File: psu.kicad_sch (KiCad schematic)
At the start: 70 parts, among them J3 Screw_Terminal_01x03, J4 Screw_Terminal_01x02, U14 ADP7182AUJZ, U15 AZ1117-ADJ, U16 AZ1117-ADJ, U19 ADP7182AUJZ, U2 AZ1117-ADJ

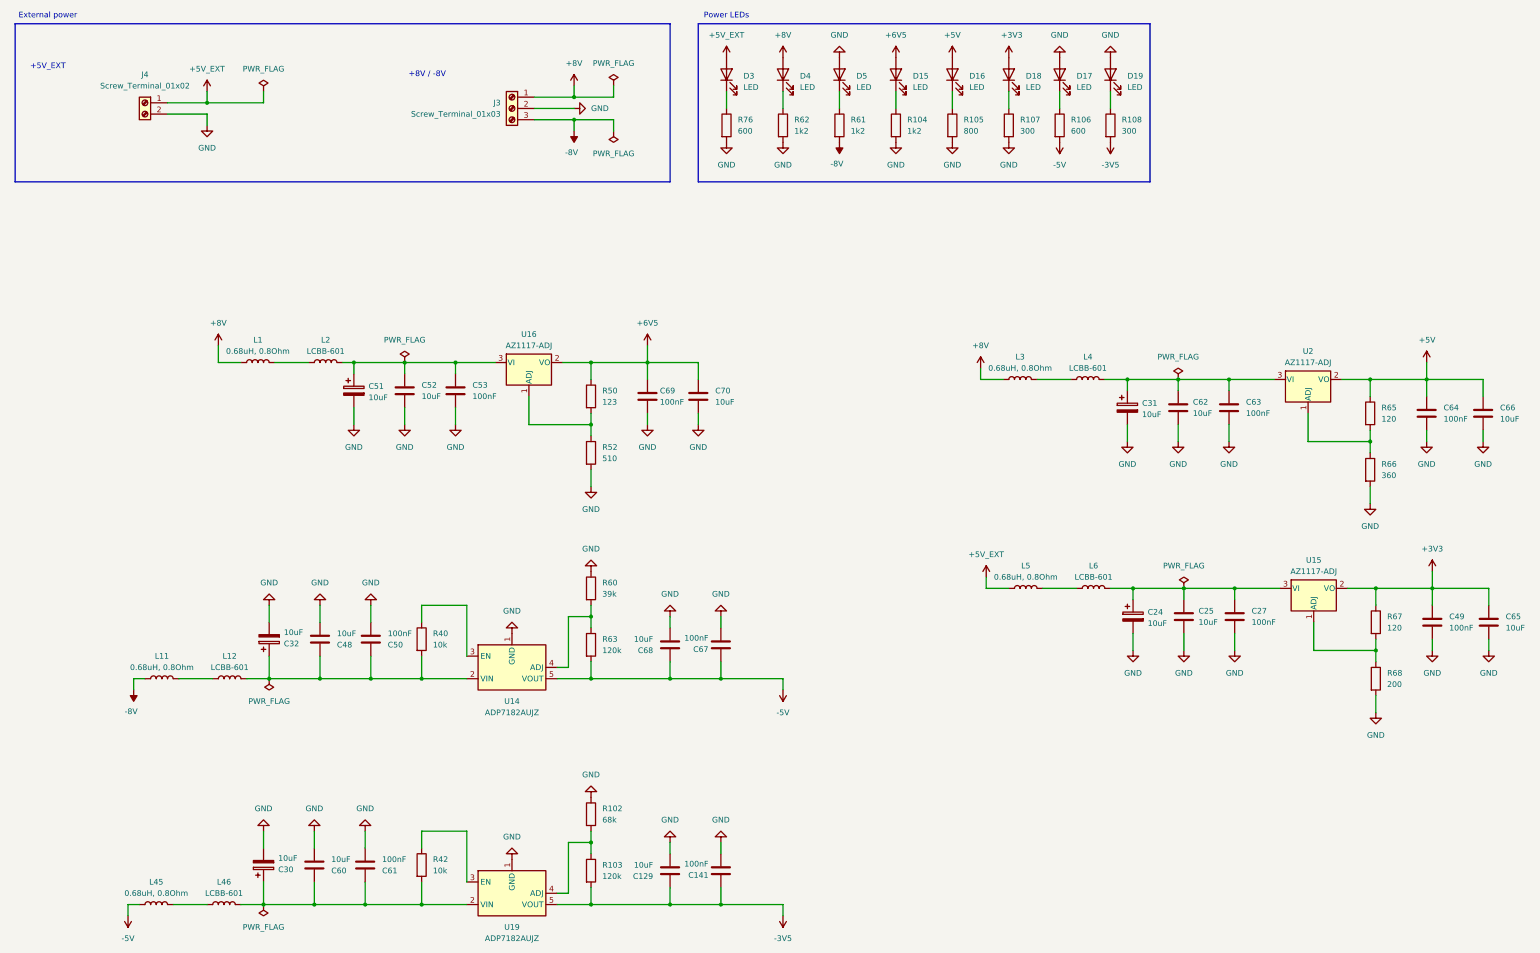
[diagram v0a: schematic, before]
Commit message: Add all footprints
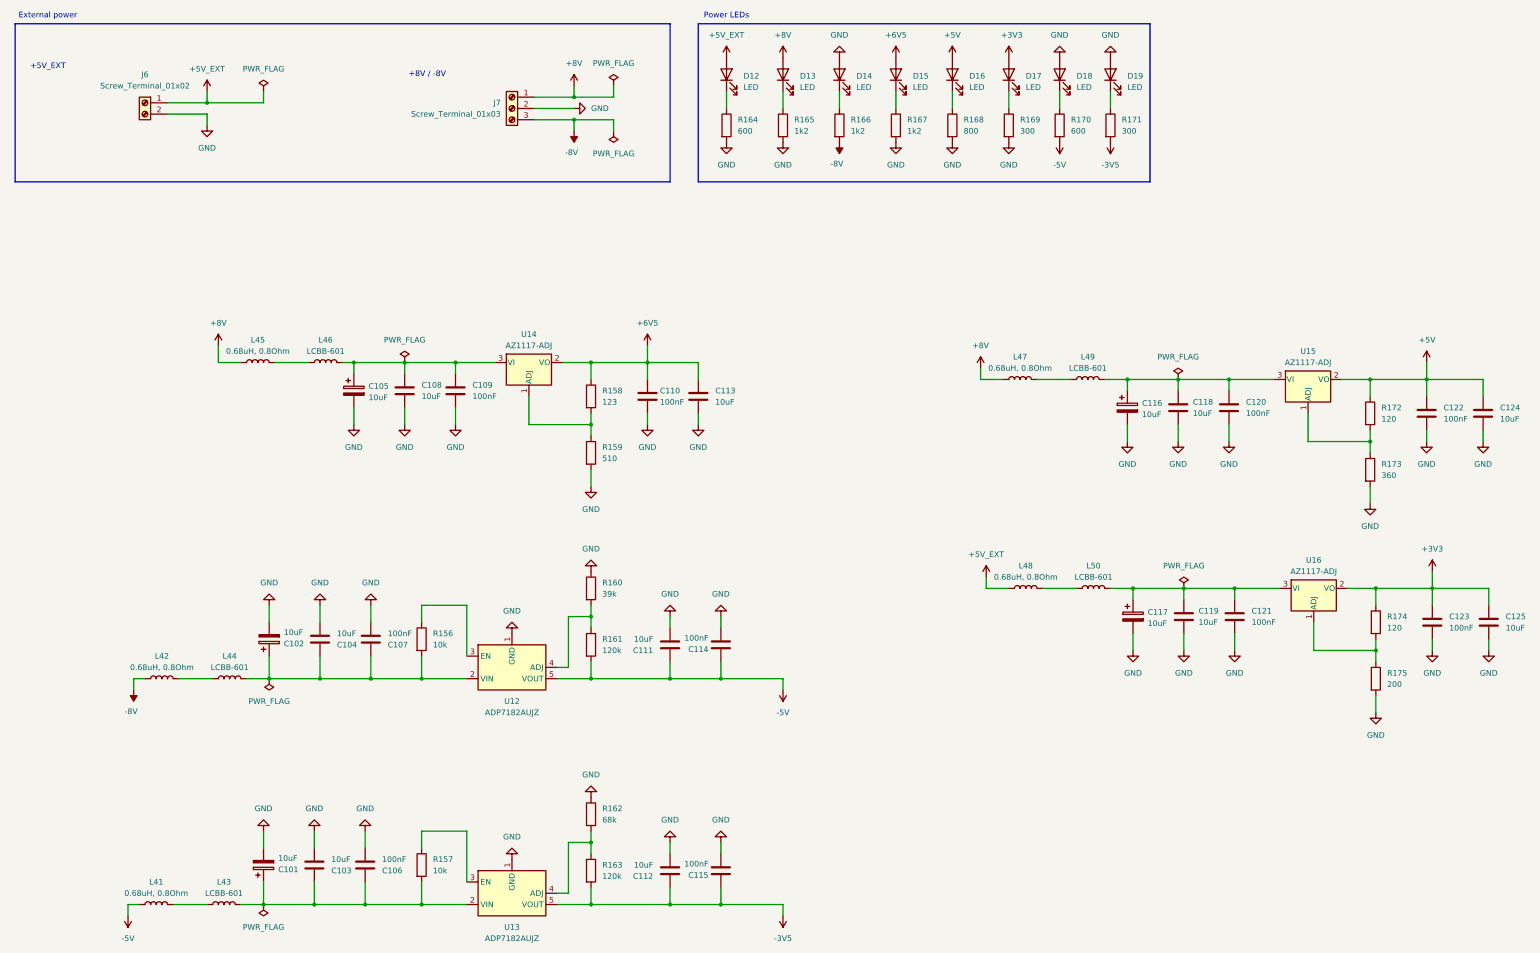
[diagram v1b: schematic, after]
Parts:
- D12: renamed from D3; footprint LED_SMD:LED_0805_2012Metric -> Diode_THT:D_DO-41_SOD81_P10.16mm_Horizontal
- D13: renamed from D4; footprint LED_SMD:LED_0805_2012Metric -> Diode_THT:D_DO-41_SOD81_P10.16mm_Horizontal
- D14: renamed from D5; footprint LED_SMD:LED_0805_2012Metric -> Diode_THT:D_DO-41_SOD81_P10.16mm_Horizontal
- J6: renamed from J4; footprint (none) -> TerminalBlock:TerminalBlock_MaiXu_MX126-5.0-02P_1x02_P5.00mm
- J7: renamed from J3; footprint (none) -> TerminalBlock:TerminalBlock_MaiXu_MX126-5.0-03P_1x03_P5.00mm
- L41: renamed from L45; footprint (none) -> Inductor_SMD:L_0805_2012Metric
- L42: renamed from L11; footprint (none) -> Inductor_SMD:L_0805_2012Metric
- L43: renamed from L46; footprint (none) -> Inductor_SMD:L_0805_2012Metric
- L44: renamed from L12; footprint (none) -> Inductor_SMD:L_0805_2012Metric
- L45: renamed from L1; footprint (none) -> Inductor_SMD:L_0805_2012Metric
- L46: renamed from L2; footprint (none) -> Inductor_SMD:L_0805_2012Metric
- L47: renamed from L3; footprint (none) -> Inductor_SMD:L_0805_2012Metric
- L48: renamed from L5; footprint (none) -> Inductor_SMD:L_0805_2012Metric
- L49: renamed from L4; footprint (none) -> Inductor_SMD:L_0805_2012Metric
- L50: renamed from L6; footprint (none) -> Inductor_SMD:L_0805_2012Metric
- U14: renamed from U16; footprint (none) -> Package_TO_SOT_SMD:SOT-89-3
- U15: renamed from U2; footprint (none) -> Package_TO_SOT_SMD:SOT-89-3
- U16: renamed from U15; footprint (none) -> Package_TO_SOT_SMD:SOT-89-3
- renumbered C30 to C101, C32 to C102, C60 to C103, C48 to C104, C51 to C105, C61 to C106, C50 to C107, C52 to C108, C53 to C109, C69 to C110, C68 to C111, C129 to C112, C70 to C113, C67 to C114, C141 to C115, C31 to C116, C24 to C117, C62 to C118, C25 to C119, C63 to C120, C27 to C121, C64 to C122, C49 to C123, C66 to C124, C65 to C125, D18 to D17, D17 to D18, R40 to R156, R42 to R157, R50 to R158, R52 to R159, R60 to R160, R63 to R161, R102 to R162, R103 to R163, R76 to R164, R62 to R165, R61 to R166, R104 to R167, R105 to R168, R107 to R169, R106 to R170, R108 to R171, R65 to R172, R66 to R173, R67 to R174, R68 to R175, U14 to U12, U19 to U13
